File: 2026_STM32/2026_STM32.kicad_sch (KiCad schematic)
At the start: 22 parts, among them J1 USB_B, J2 Conn_01x05_Pin, SW1 1825910-6, U1 SPX3819M5-L-3-3, U2 STM32C011F4P6, U3 KTD2026

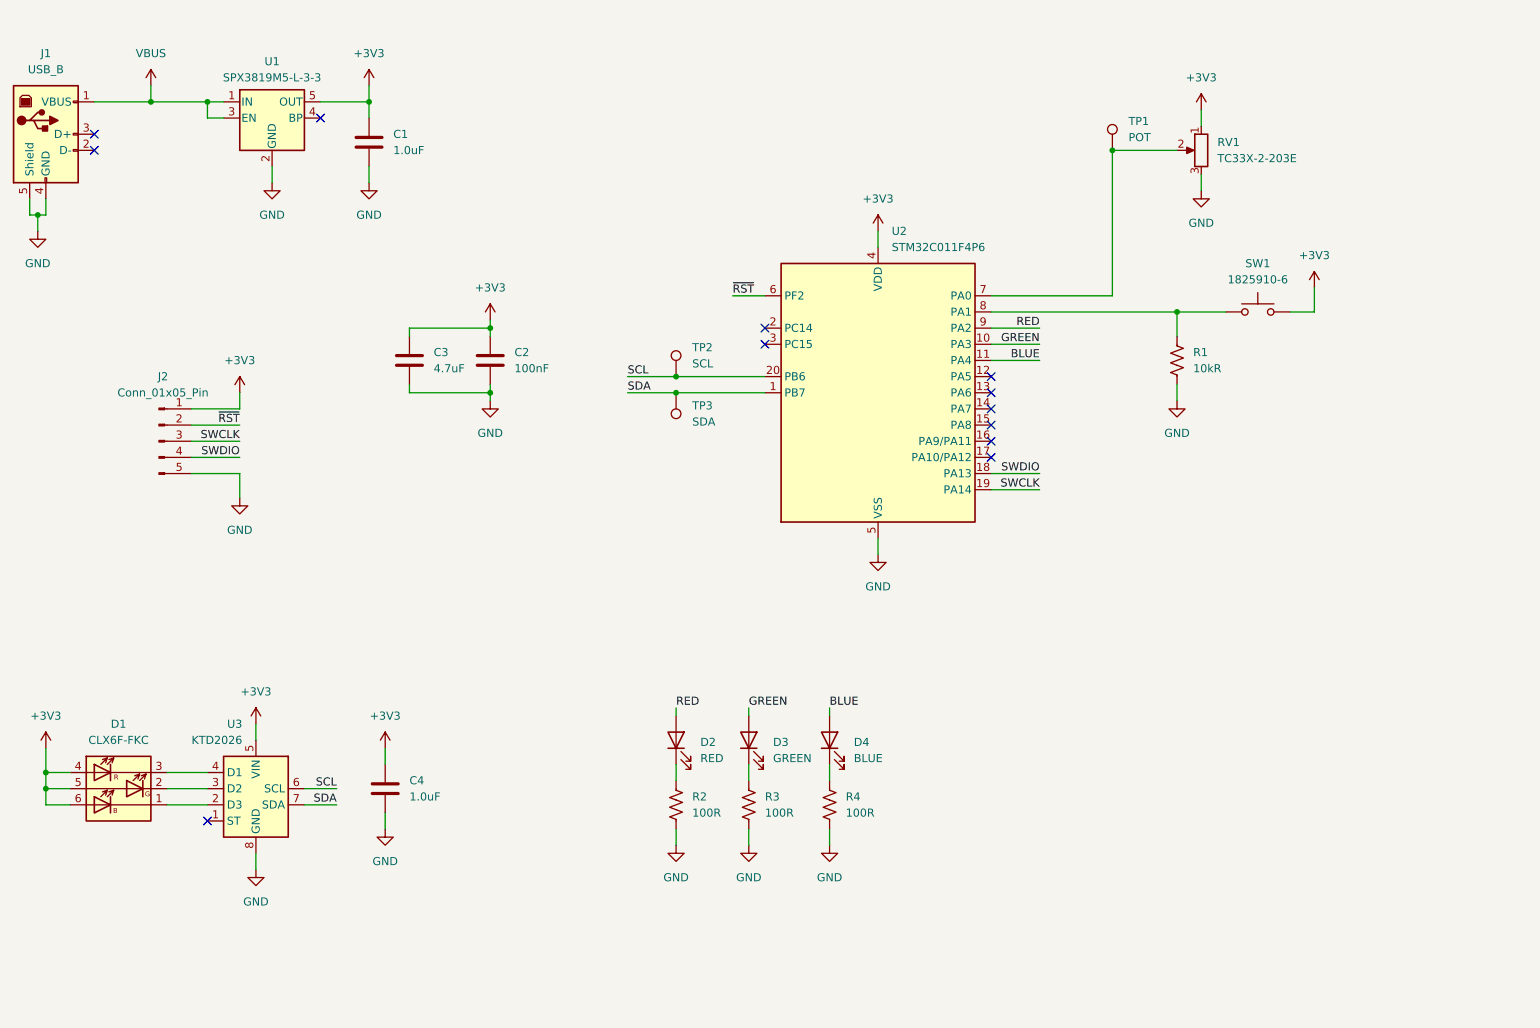
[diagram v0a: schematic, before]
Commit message: stuff
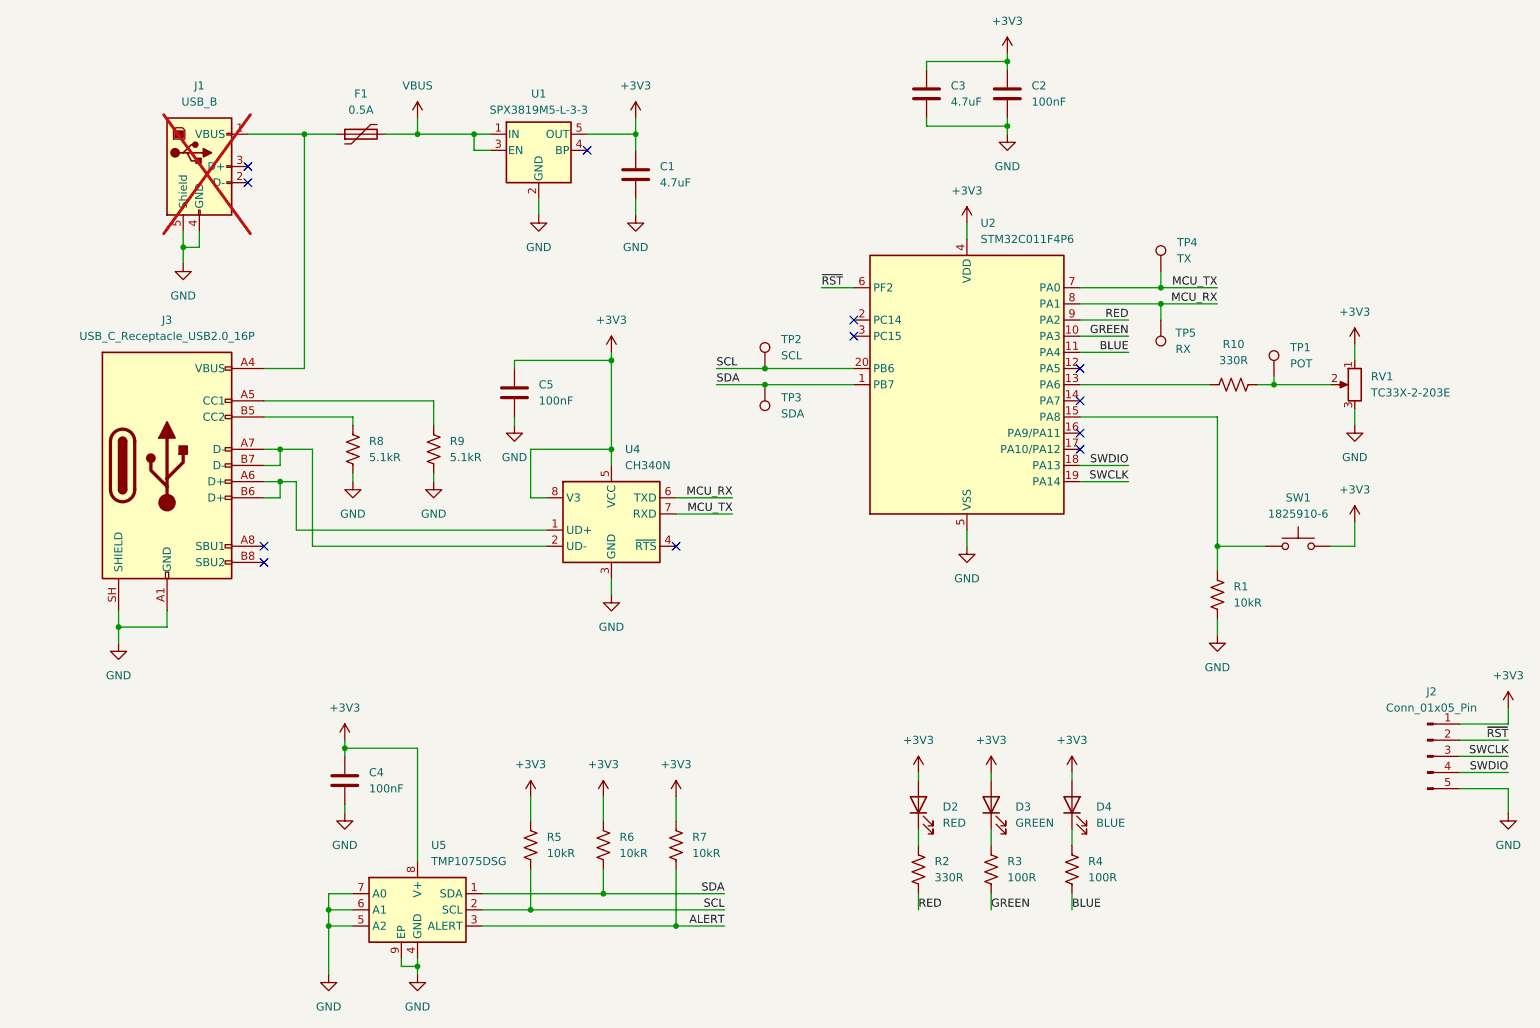
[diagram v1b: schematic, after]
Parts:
- removed D1: CLX6F-FKC, LED_SMD:LED_RGB_PLCC-6, symbol LED:CLX6F-FKC
- removed U3: KTD2026, Package_DFN_QFN:DFN-8-1EP_1.5x1.5mm_P0.4mm_EP0.7x1.2mm, symbol Driver_LED:KTD2026
- added C5: 100nF, Capacitor_SMD:C_0805_2012Metric_Pad1.18x1.45mm_HandSolder, symbol Device:C
- added F1: 0.5A, Fuse:Fuse_0805_2012Metric_Pad1.15x1.40mm_HandSolder, symbol Device:Polyfuse
- added J3: USB_C_Receptacle_USB2.0_16P, Connector_USB:USB_C_Receptacle_GCT_USB4105-xx-A_16P_TopMnt_Horizontal, symbol Connector:USB_C_Receptacle_USB2.0_16P
- added R10: 330R, Capacitor_SMD:C_0805_2012Metric_Pad1.18x1.45mm_HandSolder, symbol Device:R_US
- added R5, R6, R7: 10kR, Capacitor_SMD:C_0805_2012Metric_Pad1.18x1.45mm_HandSolder, symbol Device:R_US
- added R8, R9: 5.1kR, Capacitor_SMD:C_0805_2012Metric_Pad1.18x1.45mm_HandSolder, symbol Device:R_US
- added TP4: TX, TestPoint:TestPoint_THTPad_D2.5mm_Drill1.2mm, symbol Connector:TestPoint
- added TP5: RX, TestPoint:TestPoint_THTPad_D2.5mm_Drill1.2mm, symbol Connector:TestPoint
- added U4: CH340N, Package_SO:JEITA_SOIC-8_3.9x4.9mm_P1.27mm, symbol Interface_USB:CH340N
- added U5: TMP1075DSG, Package_SON:WSON-8-1EP_2x2mm_P0.5mm_EP0.9x1.6mm_ThermalVias, symbol Sensor_Temperature:TMP1075DSG
- C1: value 1.0uF -> 4.7uF
- C4: value 1.0uF -> 100nF
- J1: now not fitted
- R2: value 100R -> 330R
- RV1: footprint Potentiometer_SMD:Potentiometer_Bourns_TC33X_Vertical -> 2026 tutorial:PTV09A4015UB103
- SW1: LCSC (none) -> C428628
- TP1, TP2, TP3: footprint TestPoint:TestPoint_Pad_D2.5mm -> TestPoint:TestPoint_THTPad_D2.5mm_Drill1.2mm
- U2: LCSC (none) -> C7373263
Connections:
- net +3V3: now also D2.2 (A), D3.2 (A), D4.2 (A), C5.1, R5.1, R6.1, R7.1, U4.5 (VCC), U4.8 (V3), U5.8 (V+)
- net BLUE: now also R4.2; no longer D4.2 (A)
- net GND: now also C5.2, J3.A1 (GND), J3.A12 (GND), J3.B1 (GND), J3.B12 (GND), J3.SH (SHIELD), R8.2, R9.2, U4.3 (GND), U5.4 (GND), U5.5 (A2), U5.6 (A1), U5.7 (A0), U5.9 (EP); no longer R2.2, R3.2, R4.2
- net GREEN: now also R3.2; no longer D3.2 (A)
- net RED: now also R2.2; no longer D2.2 (A)
- net SCL: now also R5.2, U5.2 (SCL)
- net SDA: now also R6.2, U5.1 (SDA)
- net VBUS: now also F1.2; no longer J1.1 (VBUS)
- net at R1.1, SW1.1: now also U2.15 (PA8); no longer U2.8 (PA1)
- net at RV1.2, TP1.1: now also R10.2; no longer U2.7 (PA0)
- net at U2.13 (PA6): now also R10.1
- new net: J3.A6 (D+), J3.B6 (D+), U4.1 (UD+)
- new net: J3.A7 (D-), J3.B7 (D-), U4.2 (UD-)
- new net: F1.1, J1.1 (VBUS), J3.A4 (VBUS), J3.A9 (VBUS), J3.B4 (VBUS), J3.B9 (VBUS)
- new net: J3.A5 (CC1), R9.1
- new net: J3.B5 (CC2), R8.1
- new net ALERT: R7.2, U5.3 (ALERT)
- new net MCU_RX: TP5.1, U2.8 (PA1), U4.6 (TXD)
- new net MCU_TX: TP4.1, U2.7 (PA0), U4.7 (RXD)
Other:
- moved on the sheet: C2, C3, D2, D3, D4, J2, R2, R3, R4, TP2, TP3, U2
